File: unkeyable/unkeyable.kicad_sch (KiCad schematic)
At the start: 6 parts, among them J2 USB_C_Receptacle_USB2.0_14P, U4 NCP1117-3.3_SOT223

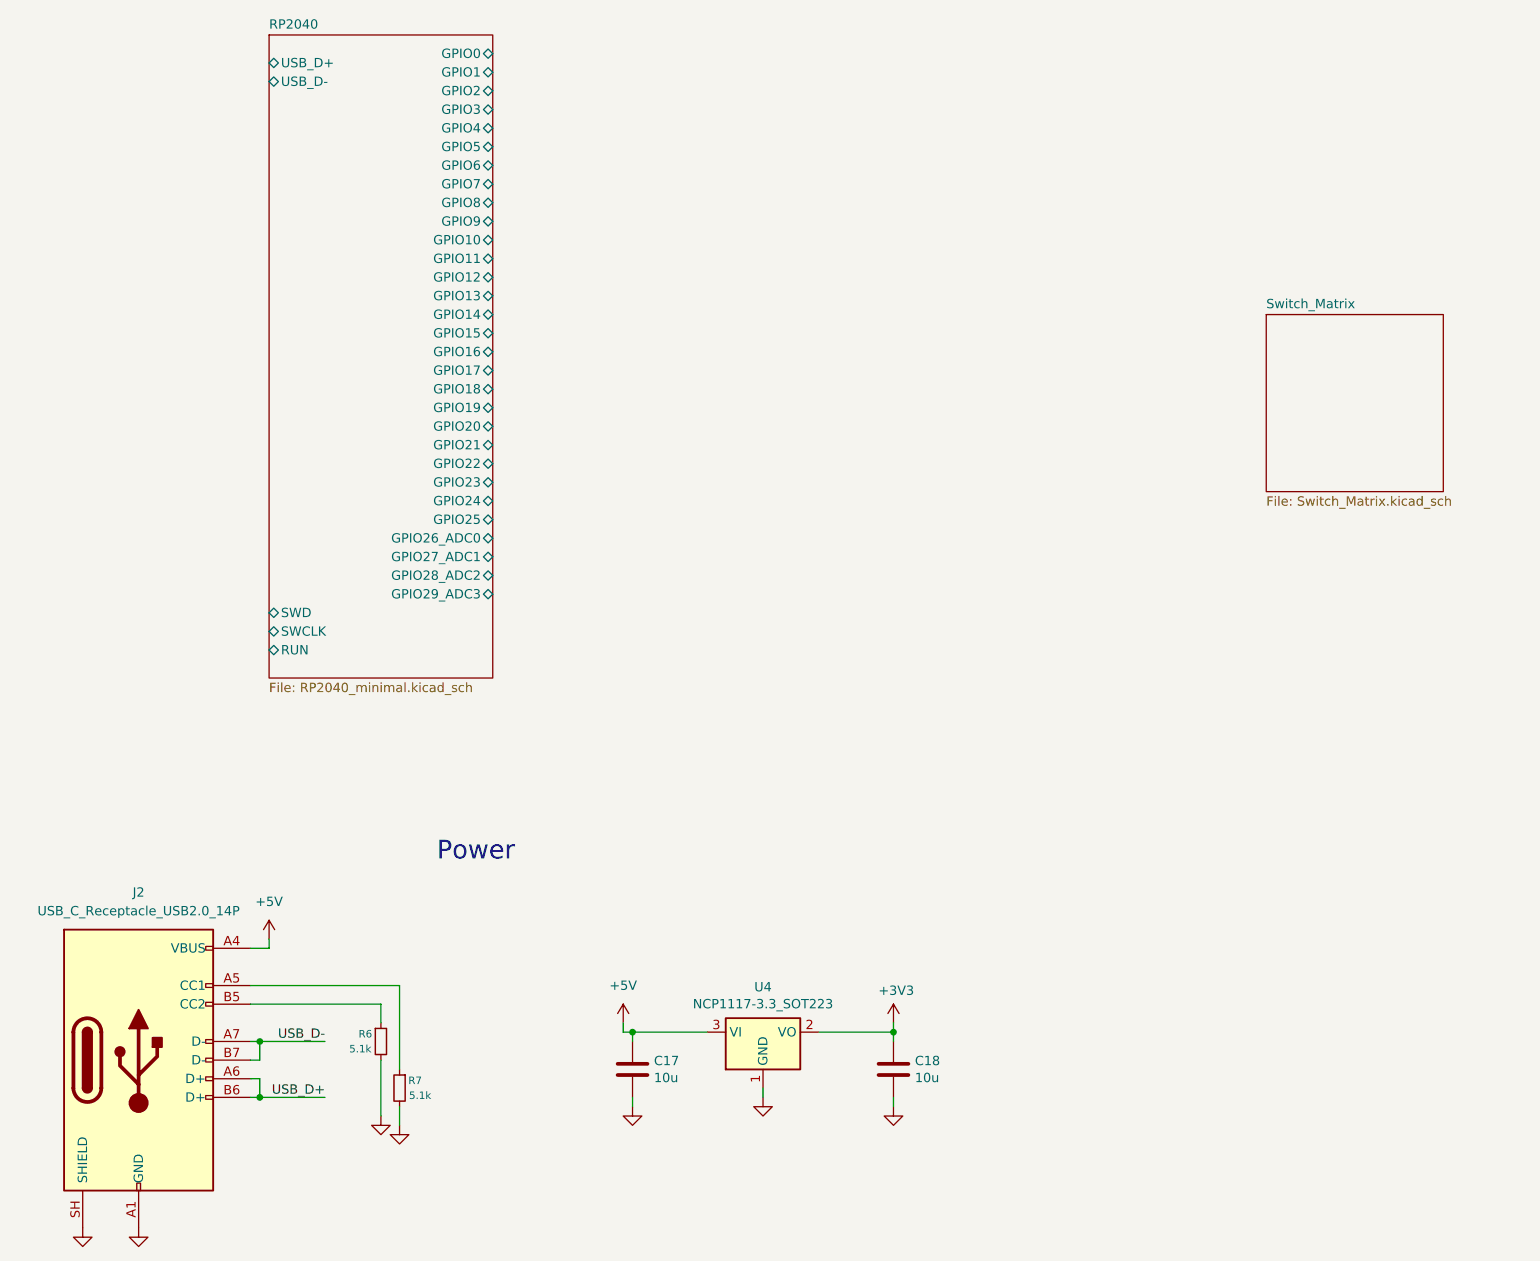
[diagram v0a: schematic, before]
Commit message: layout
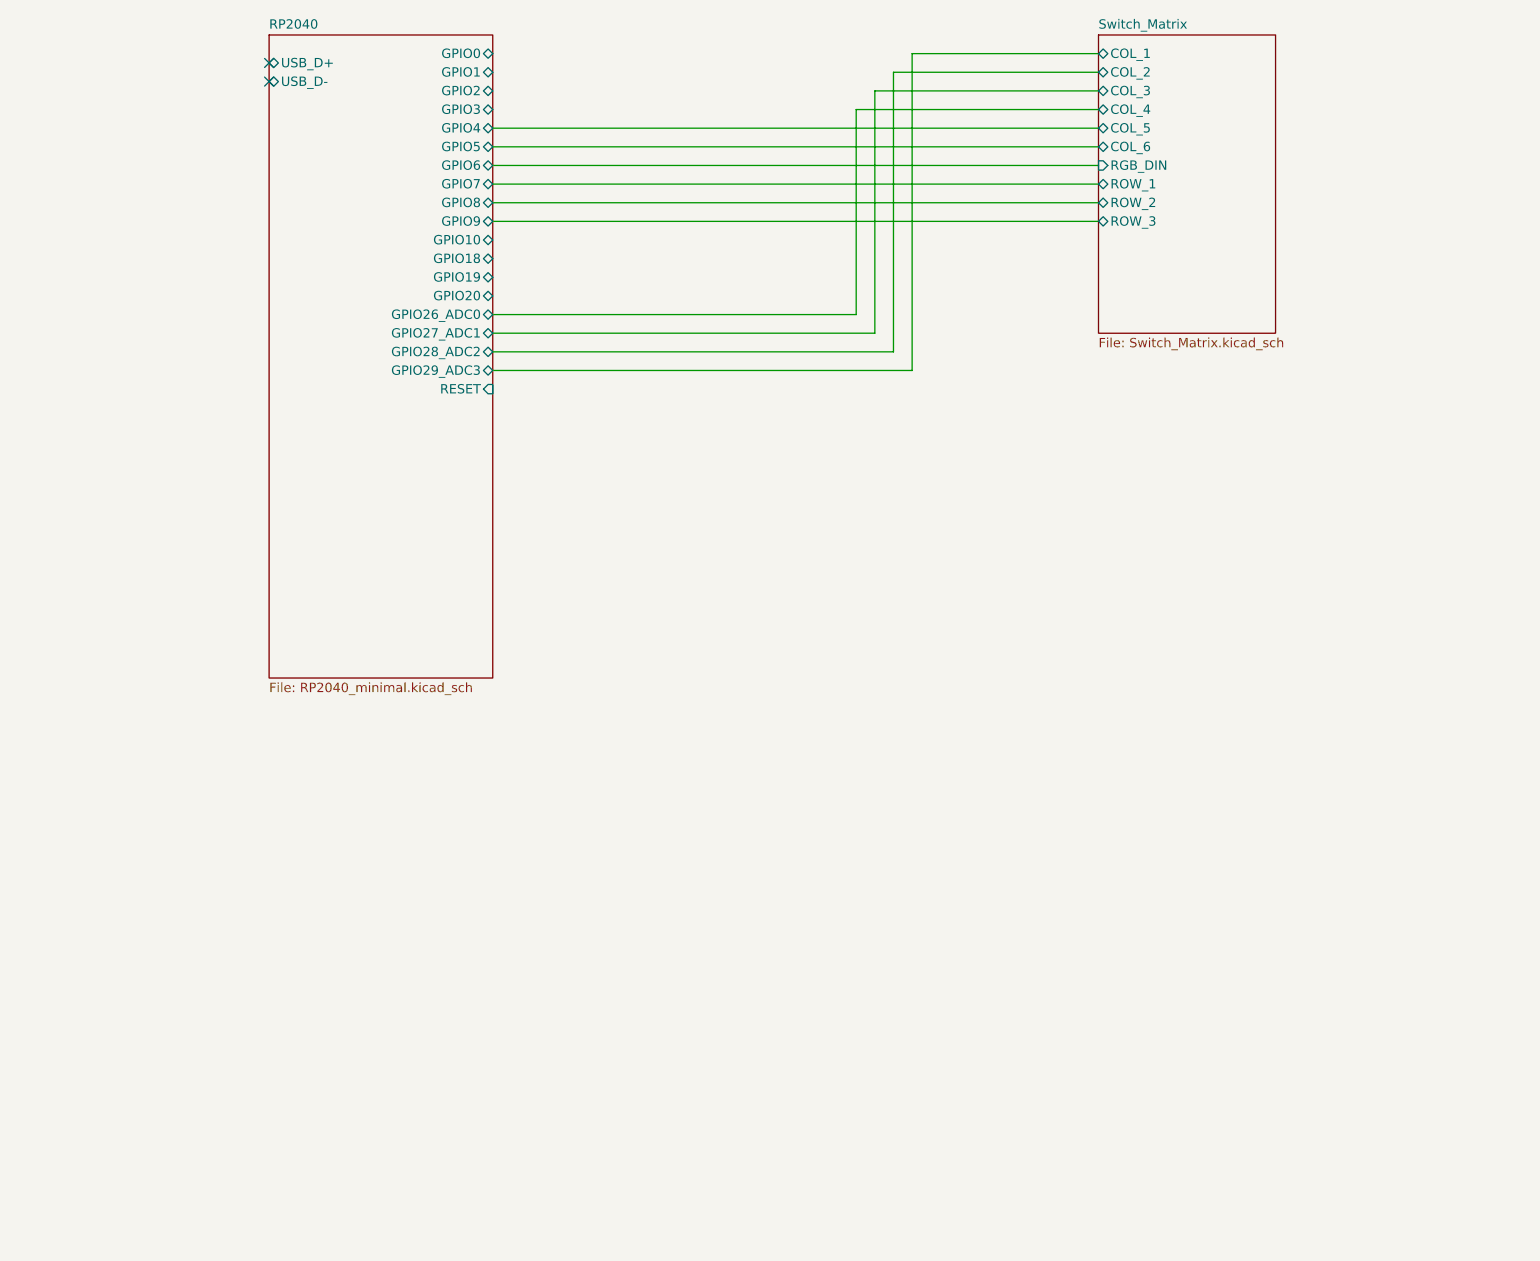
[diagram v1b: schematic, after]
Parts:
- removed C17, C18: 10u, Capacitor_SMD:C_0805_2012Metric, symbol Device:C
- removed J2: USB_C_Receptacle_USB2.0_14P, symbol Connector:USB_C_Receptacle_USB2.0_14P
- removed R6, R7: 5.1k, symbol Device:R_Small
- removed U4: NCP1117-3.3_SOT223, Package_TO_SOT_SMD:SOT-223-3_TabPin2, symbol Regulator_Linear:NCP1117-3.3_SOT223
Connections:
- no-connect marks 0 -> 2
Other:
- sheet RP2040 ports: added RESET; removed GPIO11, GPIO12, GPIO13, GPIO14, GPIO15, GPIO16, GPIO17, GPIO21, GPIO22, GPIO23, GPIO24, GPIO25, RUN, SWCLK, SWD
- sheet Switch_Matrix ports: added COL_1, COL_2, COL_3, COL_4, COL_5, COL_6, RGB_DIN, ROW_1, ROW_2, ROW_3; removed none
- note removed: "Power"
